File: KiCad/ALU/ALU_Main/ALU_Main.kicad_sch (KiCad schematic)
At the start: 14 parts, among them J1 Conn_01x02_Socket, J2 Conn_01x04_Socket, J3 Conn_01x05_Socket, J4 Conn_01x16_Socket, J5 Conn_01x16_Socket, J8 Conn_01x16_Socket, U1 74LS181, U2 74LS181, U3 74LS181, U4 74LS181

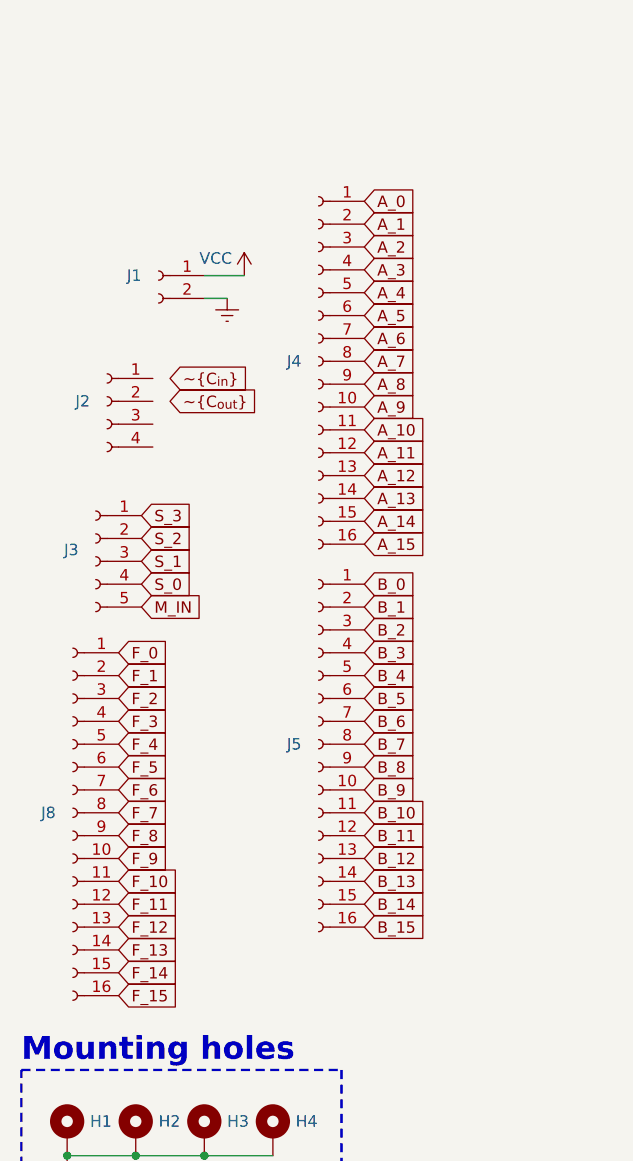
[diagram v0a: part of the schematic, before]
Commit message: .
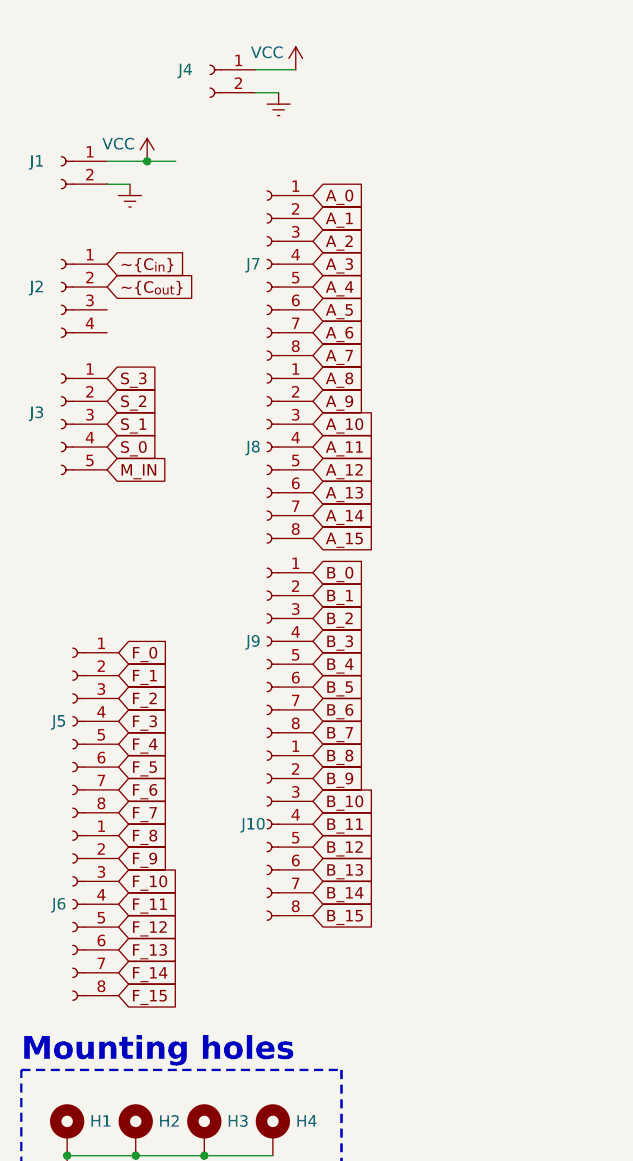
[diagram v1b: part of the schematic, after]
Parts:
- removed J4, J5, J8: Conn_01x16_Socket, Connector_IDC:IDC-Header_2x08_P2.54mm_Horizontal, symbol Connector:Conn_01x16_Socket
- added J10, J5, J6, J7, J8, J9: Conn_01x08_Socket, Connector_JST:JST_XH_S8B-XH-A-1_1x08_P2.50mm_Horizontal, symbol Connector:Conn_01x08_Socket
- added J4: Conn_01x02_Socket, Connector_JST:JST_XH_S2B-XH-A-1_1x02_P2.50mm_Horizontal, symbol Connector:Conn_01x02_Socket
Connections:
- net A_0: now also J7.1 (Pin_1)
- net A_1: now also J7.2 (Pin_2)
- net A_10: now also J8.3 (Pin_3)
- net A_11: now also J8.4 (Pin_4)
- net A_12: now also J8.5 (Pin_5)
- net A_13: now also J8.6 (Pin_6)
- net A_14: now also J8.7 (Pin_7)
- net A_15: now also J8.8 (Pin_8)
- net A_2: now also J7.3 (Pin_3)
- net A_3: now also J7.4 (Pin_4)
- net A_4: now also J7.5 (Pin_5)
- net A_5: now also J7.6 (Pin_6)
- net A_6: now also J7.7 (Pin_7)
- net A_7: now also J7.8 (Pin_8)
- net A_8: now also J8.1 (Pin_1)
- net A_9: now also J8.2 (Pin_2)
- net B_0: now also J9.1 (Pin_1)
- net B_1: now also J9.2 (Pin_2)
- net B_10: now also J10.3 (Pin_3)
- net B_11: now also J10.4 (Pin_4)
- net B_12: now also J10.5 (Pin_5)
- net B_13: now also J10.6 (Pin_6)
- net B_14: now also J10.7 (Pin_7)
- net B_15: now also J10.8 (Pin_8)
- net B_2: now also J9.3 (Pin_3)
- net B_3: now also J9.4 (Pin_4)
- net B_4: now also J9.5 (Pin_5)
- net B_5: now also J9.6 (Pin_6)
- net B_6: now also J9.7 (Pin_7)
- net B_7: now also J9.8 (Pin_8)
- net B_8: now also J10.1 (Pin_1)
- net B_9: now also J10.2 (Pin_2)
- net F_0: now also J5.1 (Pin_1)
- net F_1: now also J5.2 (Pin_2)
- net F_10: now also J6.3 (Pin_3)
- net F_11: now also J6.4 (Pin_4)
- net F_12: now also J6.5 (Pin_5)
- net F_13: now also J6.6 (Pin_6)
- net F_14: now also J6.7 (Pin_7)
- net F_15: now also J6.8 (Pin_8)
- net F_2: now also J5.3 (Pin_3)
- net F_3: now also J5.4 (Pin_4)
- net F_4: now also J5.5 (Pin_5)
- net F_5: now also J5.6 (Pin_6)
- net F_6: now also J5.7 (Pin_7)
- net F_7: now also J5.8 (Pin_8)
- net F_8: now also J6.1 (Pin_1)
- net F_9: now also J6.2 (Pin_2)
- net GND: now also J4.2 (Pin_2)
- net VCC: now also J4.1 (Pin_1)
- net ~{C_{in}}: now also J2.1 (Pin_1)
- net ~{C_{out}}: now also J2.2 (Pin_2)
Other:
- moved on the sheet: J1, J2, J3
